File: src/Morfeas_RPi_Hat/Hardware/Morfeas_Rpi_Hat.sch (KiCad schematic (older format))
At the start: 47 parts, among them J1 Power IN, J2 RPi_header, J3 CAN0_Power+, J4 CAN1_Power+, J5 RS_232, Q1 SUM110P06, Q2 SUM110P06, U1 DS3231, U2 TSR2-2450, U3 TLV70433, U4 SP3232, U5 24AA08, U6 MAX9611, U7 MAX9611

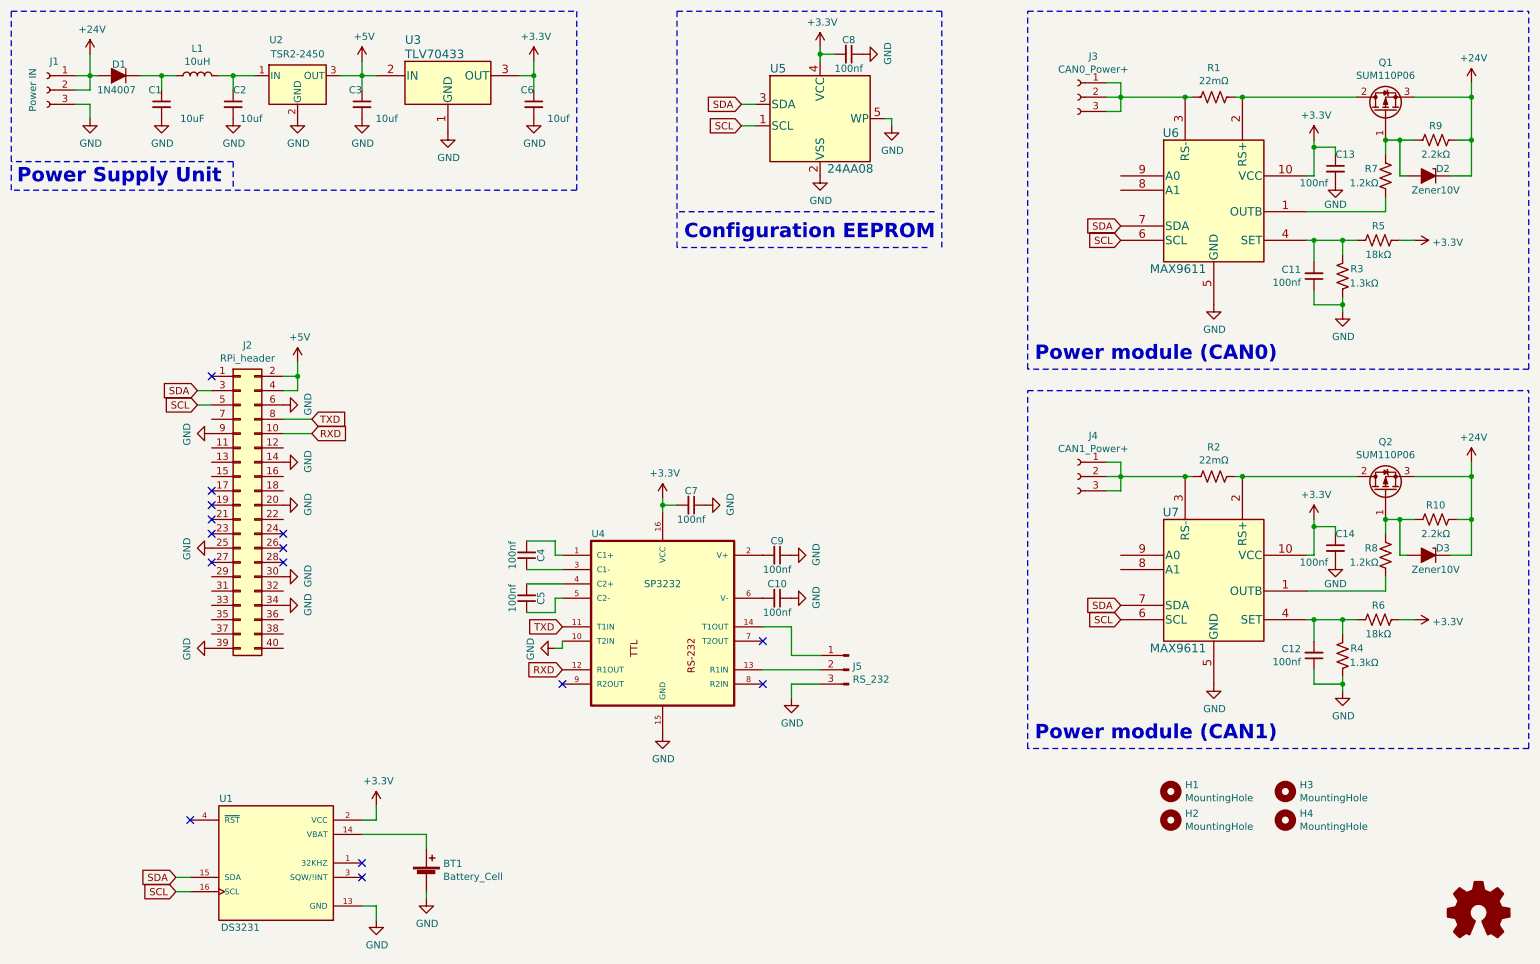
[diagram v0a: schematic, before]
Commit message: Update
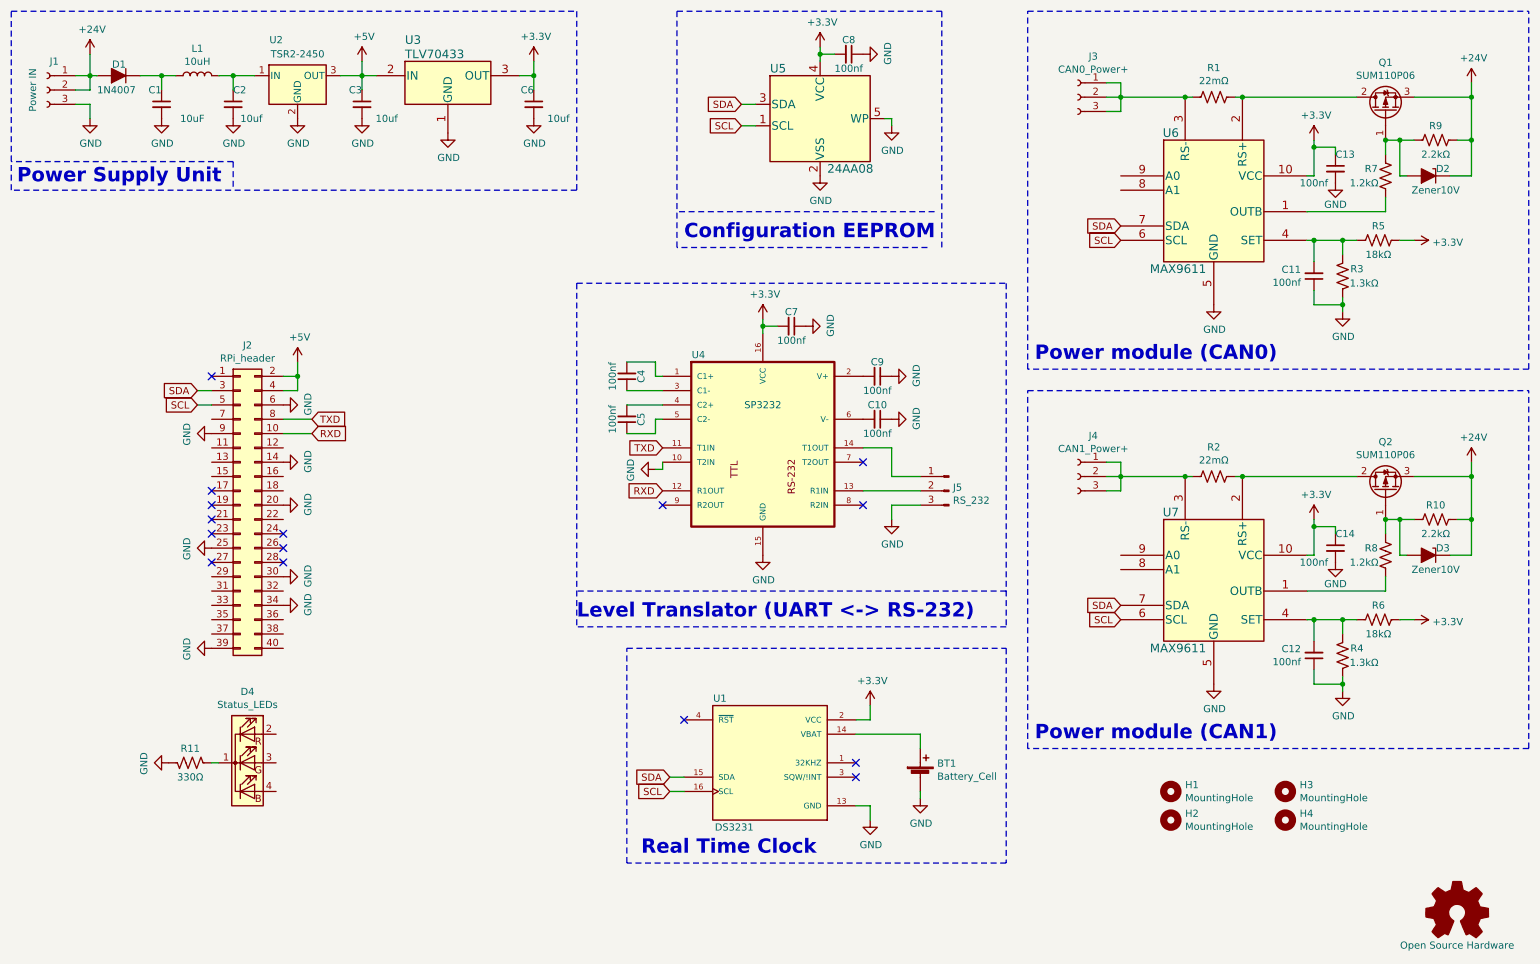
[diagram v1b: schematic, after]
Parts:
- added D4: Status_LEDs, LEDs:LED_D5.0mm-4, symbol Device:LED_CRGB
- added R11: 330Ω, Resistors_SMD:R_1206, symbol Device:R_US
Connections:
- net GND: now also R11.2
- new net: D4.1 (K), R11.1
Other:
- note added: "Level Translator (UART <-> RS-232)"
- note added: "Real Time Clock"
- moved on the sheet: BT1, C10, C4, C5, C7, C9, J5, U1, U4

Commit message: Update
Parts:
- D4: footprint LEDs:LED_D5.0mm-4 -> LED_THT:LED_D5.0mm-4_RGB
- R11: footprint Resistors_SMD:R_1206 -> Resistor_SMD:R_1206_3216Metric
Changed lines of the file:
@@
 F 0 "D4" H 2200 6297 50  0000 C CNN
 F 1 "Status_LEDs" H 2200 6206 50  0000 C CNN
-F 2 "LEDs:LED_D5.0mm-4" H 2200 5750 50  0001 C CNN
+F 2 "LED_THT:LED_D5.0mm-4_RGB" H 2200 5750 50  0001 C CNN
 F 3 "~" H 2200 5750 50  0001 C CNN
 	1    2200 5800
@@
 F 0 "R11" V 1900 5800 50  0000 C CNN
 F 1 "330Ω" V 1700 5800 50  0000 C CNN
-F 2 "Resistors_SMD:R_1206" V 1840 5790 50  0001 C CNN
+F 2 "Resistor_SMD:R_1206_3216Metric" V 1840 5790 50  0001 C CNN
 F 3 "~" H 1800 5800 50  0001 C CNN
 	1    1800 5800

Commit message: Update
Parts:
- J5: footprint Connectors_Molex:Molex_KK-6410-03_03x2.54mm_Straight -> Connector_PinHeader_2.54mm:PinHeader_1x03_P2.54mm_Horizontal
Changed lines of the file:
@@
 F 0 "J5" H 7072 3924 50  0000 R CNN
 F 1 "RS_232" H 7072 3833 50  0000 R CNN
-F 2 "Connectors_Molex:Molex_KK-6410-03_03x2.54mm_Straight" H 7100 3900 50  0001 C CNN
+F 2 "Connector_PinHeader_2.54mm:PinHeader_1x03_P2.54mm_Horizontal" H 7100 3900 50  0001 C CNN
 F 3 "~" H 7100 3900 50  0001 C CNN
 	1    7100 3900
